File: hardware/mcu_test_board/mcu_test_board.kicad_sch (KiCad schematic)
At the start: 28 parts, among them CN1 KF2EDGR-2.54-2P, CN2 KF2EDGR-2.54-2P, CN3 SM04B-SRSS-TB (LF)(SN), CN4 KF2EDGR-2.54-4P, J1 Conn_ARM_SWD_TagConnect_TC203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, SW1 DSHP04TSGER, U2 LD39050PU33R, U4 STM32G431KBT6TR, X1 NX2016SA-16MHZ-EXS00A-CS07826

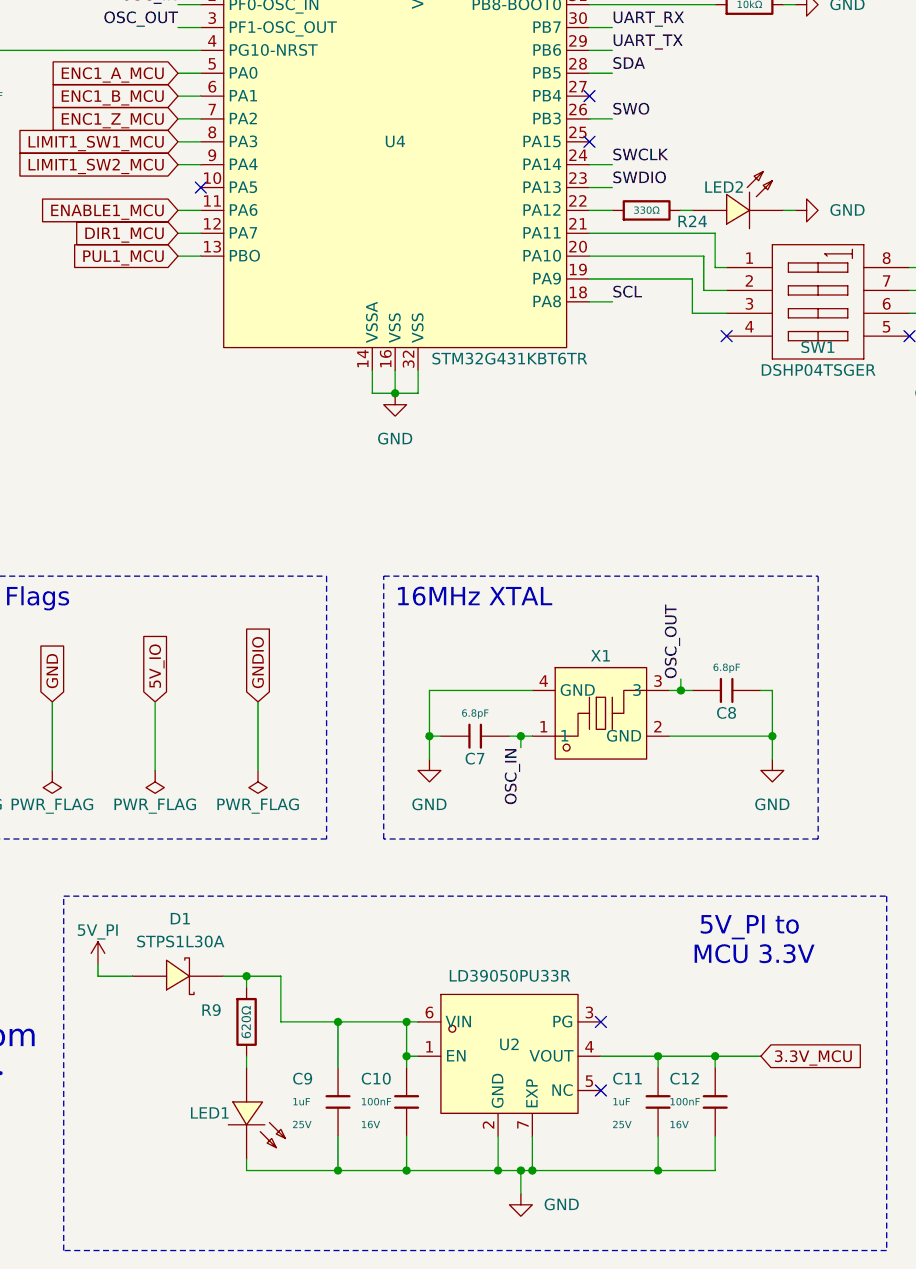
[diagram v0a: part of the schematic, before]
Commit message: Adjusting parts
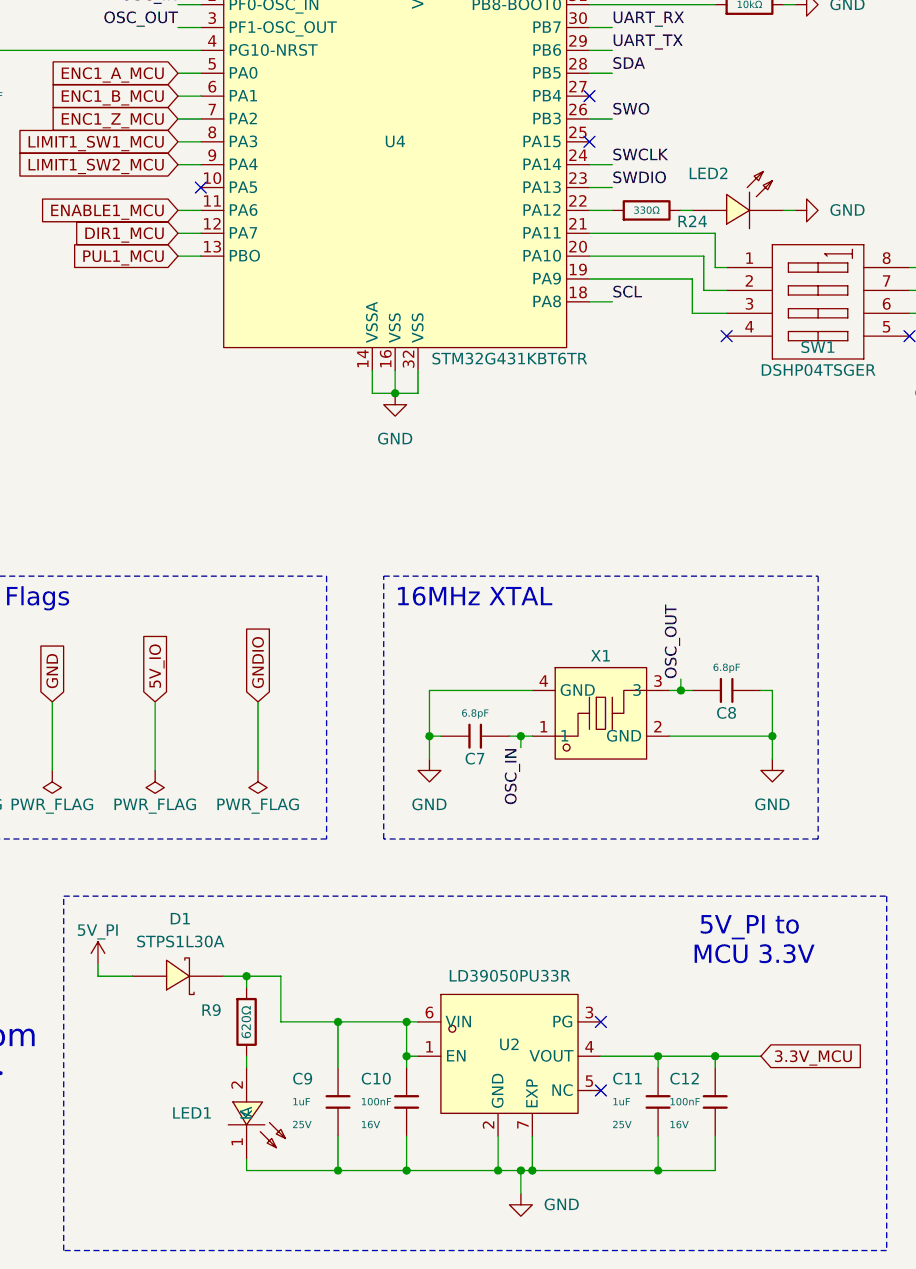
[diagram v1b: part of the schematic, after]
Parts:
- removed LED1, LED2: 19-213SYGC/S530-E2/TR8, MyParts:LED-SMD_L1.6-W0.8-FD_GREEN, symbol MyParts:19-213SYGC_S530-E2_TR8
- added LED1, LED2: LTST-S270KGKT, MyParts:LED-SMD_L1.7-W0.6-RD, symbol MyParts:LTST-S270KGKT
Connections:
- net GND: now also LED1.1 (K), LED2.1 (K)
- net at R9.2: now also LED1.2 (A)
- net at R24.2: now also LED2.2 (A)
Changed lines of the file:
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@@
-	)
-	(symbol
-		(lib_id "MyParts:19-213SYGC_S530-E2_TR8")
-		(at 118.11 77.47 0)
-		(unit 1)
-		(exclude_from_sim no)
-		(in_bom yes)
-		(on_board yes)
-		(dnp no)
-		(property "Reference" "LED2"
-			(at 114.3 74.93 0)
-			(effects
-				(font
-					(size 1.27 1.27)
-				)
-				(justify left)
-			)
-		)
-		(property "Value" "19-213SYGC/S530-E2/TR8"
-			(at 119.38 71.12 0)
-			(effects
-				(font
-					(size 1.27 1.27)
-				)
-				(hide yes)
-			)
-		)
-		(property "Footprint" "MyParts:LED-SMD_L1.6-W0.8-FD_GREEN"
-			(at 118.11 85.09 0)
-			(effects
-				(font
-					(size 1.27 1.27)
-				)
-				(hide yes)
-			)
-		)
-		(property "Datasheet" "https://lcsc.com/product-detail/New-Arrivals_Everlight-Elec-19-213SYGC-S530-E2-TR8_C409444.html"
-			(at 118.11 87.63 0)
-			(effects
-				(font
-					(size 1.27 1.27)
-				)
-				(hide yes)
-			)
-		)
-		(property "Description" ""
-			(at 118.11 77.47 0)
-			(effects
-				(font
-					(size 1.27 1.27)
-				)
-				(hide yes)
-			)
-		)
-		(property "LCSC Part" "C409444"
-			(at 118.11 90.17 0)
-			(effects
-				(font
-					(size 1.27 1.27)
-				)
-				(hide yes)
-			)
-		)
-		(pin "2"
-		)
-		(pin "1"
-		)
-		(instances
-			(project "mcu_test_board"
-				(path "/262d8f76-cfc1-4cac-8f67-8c56cd47dd59"
-					(reference "LED2")
-					(unit 1)
-				)
-			)
-		)
 	)
 	(symbol
@@
 	)
 	(symbol
+		(lib_name "LTST-S270KGKT_1")
+		(lib_id "MyParts:LTST-S270KGKT")
+		(at 118.11 77.47 0)
+		(mirror y)
+		(unit 1)
+		(exclude_from_sim no)
+		(in_bom yes)
+		(on_board yes)
+		(dnp no)
+		(property "Reference" "LED2"
+			(at 117.094 73.406 0)
+			(effects
+				(font
+					(size 1.27 1.27)
+				)
+				(justify left)
+			)
+		)
+		(property "Value" "LTST-S270KGKT"
+			(at 120.6499 81.28 90)
+			(effects
+				(font
+					(size 1.27 1.27)
+				)
+				(justify right)
+				(hide yes)
+			)
+		)
+		(property "Footprint" "MyParts:LED-SMD_L1.7-W0.6-RD"
+			(at 118.11 85.09 0)
+			(effects
+				(font
+					(size 1.27 1.27)
+				)
+				(hide yes)
+			)
+		)
+		(property "Datasheet" "https://lcsc.com/product-detail/Light-Emitting-Diodes-LED_SMD-green_C125113.html"
+			(at 118.11 87.63 0)
+			(effects
+				(font
+					(size 1.27 1.27)
+				)
+				(hide yes)
+			)
+		)
+		(property "Description" ""
+			(at 118.11 77.47 0)
+			(effects
+				(font
+					(size 1.27 1.27)
+				)
+				(hide yes)
+			)
+		)
+		(property "LCSC Part" "C125113"
+			(at 118.11 90.17 0)
+			(effects
+				(font
+					(size 1.27 1.27)
+				)
+				(hide yes)
+			)
+		)
+		(pin "2"
+		)
+		(pin "1"
+		)
+		(instances
+			(project "mcu_test_board"
+				(path "/262d8f76-cfc1-4cac-8f67-8c56cd47dd59"
+					(reference "LED2")
+					(unit 1)
+				)
+			)
+		)
+	)
+	(symbol
 		(lib_id "MyParts:NX2016SA-16MHZ-EXS00A-CS07826")
 		(at 102.87 133.35 0)
@@
 	)
 	(symbol
-		(lib_id "MyParts:19-213SYGC_S530-E2_TR8")
+		(lib_id "MyParts:LTST-S270KGKT")
 		(at 63.5 177.8 270)
+		(mirror x)
 		(unit 1)
 		(exclude_from_sim no)
@@
 		(dnp no)
 		(property "Reference" "LED1"
-			(at 57.15 177.8 90)
-			(effects
-				(font
-					(size 1.27 1.27)
-				)
-				(justify left)
-			)
-		)
-		(property "Value" "19-213SYGC/S530-E2/TR8"
-			(at 69.85 179.07 0)
-			(effects
-				(font
-					(size 1.27 1.27)
-				)
-				(hide yes)
-			)
-		)
-		(property "Footprint" "MyParts:LED-SMD_L1.6-W0.8-FD_GREEN"
+			(at 59.69 177.7999 90)
+			(effects
+				(font
+					(size 1.27 1.27)
+				)
+				(justify right)
+			)
+		)
+		(property "Value" "LTST-S270KGKT"
+			(at 59.69 180.3399 90)
+			(effects
+				(font
+					(size 1.27 1.27)
+				)
+				(justify right)
+				(hide yes)
+			)
+		)
+		(property "Footprint" "MyParts:LED-SMD_L1.7-W0.6-RD"
 			(at 55.88 177.8 0)
 			(effects
@@
 			)
 		)
-		(property "Datasheet" "https://lcsc.com/product-detail/New-Arrivals_Everlight-Elec-19-213SYGC-S530-E2-TR8_C409444.html"
+		(property "Datasheet" "https://lcsc.com/product-detail/Light-Emitting-Diodes-LED_SMD-green_C125113.html"
 			(at 53.34 177.8 0)
 			(effects
@@
 			)
 		)
-		(property "LCSC Part" "C409444"
+		(property "LCSC Part" "C125113"
 			(at 50.8 177.8 0)
 			(effects
@@
 		)
 		(instances
-			(project "mcu_test_board"
+			(project ""
 				(path "/262d8f76-cfc1-4cac-8f67-8c56cd47dd59"
 					(reference "LED1")
